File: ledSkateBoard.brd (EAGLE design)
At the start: 24.9 x 43.3 mm, 14 parts, among them J1 JST, U2 USD-SOCKETNEW, U4 MIC2505 3.3

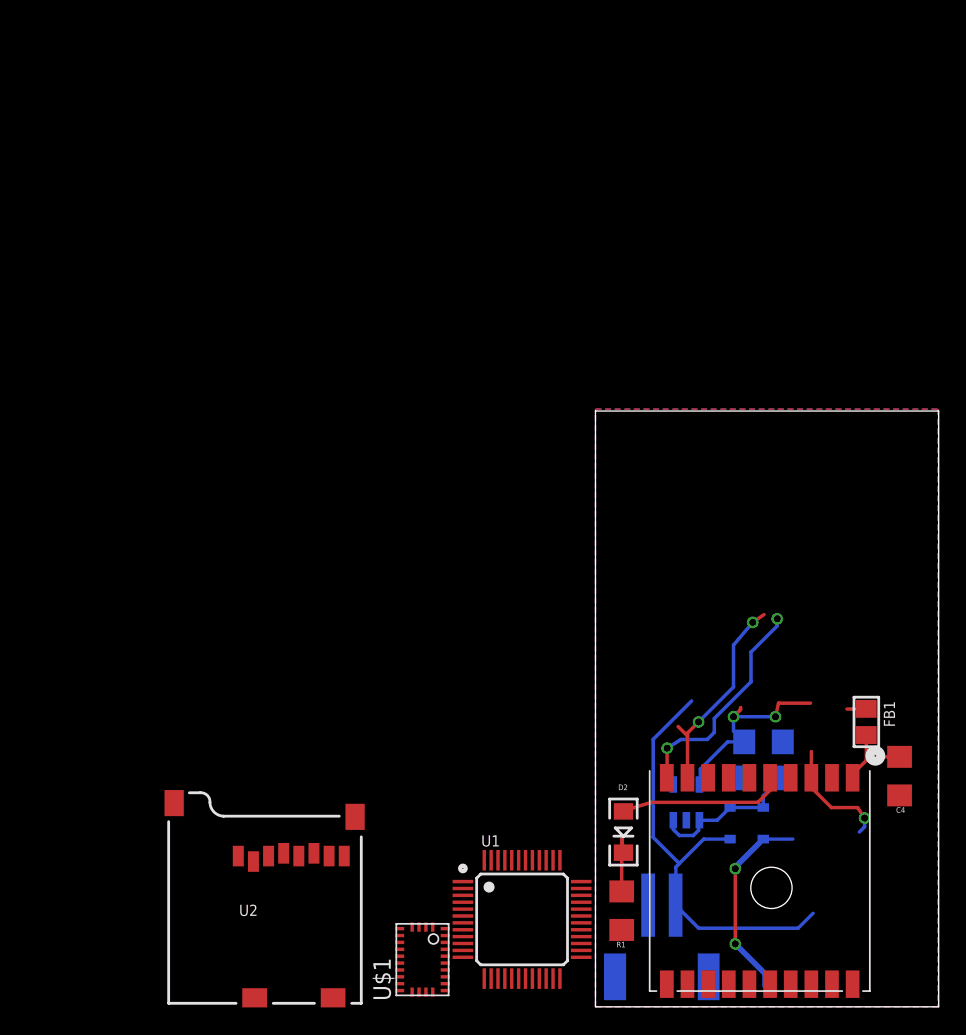
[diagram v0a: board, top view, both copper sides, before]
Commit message: faileld attempt
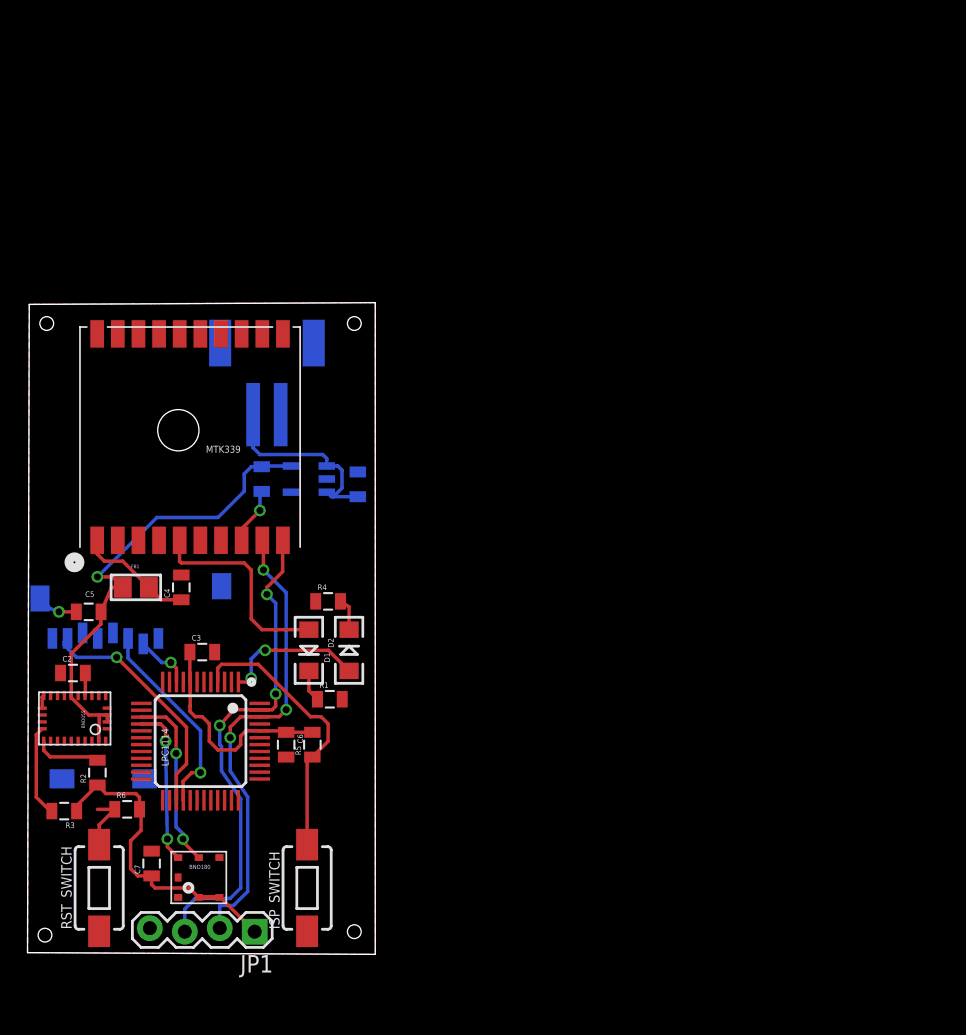
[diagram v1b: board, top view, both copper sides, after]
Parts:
- removed D3, D4: PMEG4005EJ, SparkFun-DiscreteSemi:SOD-323
- removed U1: (no value), microbuilder:LQFP48
- removed U2: USD-SOCKETNEW, SparkFun-Connectors:MICRO-SD-SOCKET-PP
- removed U3: (no value), adafruit:FGPMMOPA6H
- added BNO055: BNO055A, BNO055:BNO055
- added BNO180: BMP180, SparkFun-Sensors:BMP180
- added C2, C3, C6, C7: 10uF, SparkFun-Passives:0805
- added C5: .1uF, SparkFun-Passives:0805
- added D1: PURPLE, SparkFun-LED:LED-1206
- added ISP_SWITCH, RST_SWITCH: (no value), SparkFun-Electromechanical:TACTILE-SWITCH-1101NE
- added JP1: (no value), SparkFun-Connectors:1X04_LOCK
- added LPC1114: (no value), microbuilder:LQFP48
- added MTK339: (no value), adafruit:FGPMMOPA6H
- added R2, R3, R5, R6: 10K, SparkFun-Passives:0805
- added R4: 330, SparkFun-Passives:0805
- C14, C15, C4: device SparkFun-Capacitors:1206 -> SparkFun-Passives:0805
- R1: device SparkFun-Passives:1206 -> SparkFun-Passives:0805
- U$1: value BNO055A -> MICROSD; device BNO055:BNO055 -> adafruit:MICROSD
- moved FB1 54.0 mm to (10.4, 30.0), turned to 180 degrees
- moved C4 54.0 mm to (13.7, 30.0), turned to 90 degrees
- moved J1 51.7 mm to (19.9, 46.2), turned to 0 degrees
- moved C15 41.2 mm to (19.6, 37.8), turned to 90 degrees
- moved C14 36.3 mm to (26.5, 37.5), turned to 270 degrees
- moved U4 36.1 mm to (23.0, 37.8), turned to 270 degrees
- moved U$1 30.9 mm to (3.05, 15.6), flipped to the bottom, turned to 180 degrees
- moved D2 26.4 mm to (23.0, 25.4)
- moved R1 26.2 mm to (24.5, 21.8), turned to 0 degrees
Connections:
- removed net 5V: D3.A
- removed net GPS_RX: U1.47, U3.P$10
- removed net GPS_TX: U1.46, U3.P$9
- removed net N$10: C14.2, D3.C, D4.C, U4.1, U4.3
- removed net VDD(3.3V): U1.44
- removed net VDD(IO): U1.8
- removed net VSS(IO): U1.5
- new net BNO_INT: BNO055.14, LPC1114.14
- new net ISP: ISP_SWITCH.2, LPC1114.4, R5.1
- new net LPC_RX: JP1.2, LPC1114.46, MTK339.P$9
- new net LPC_TX: JP1.3, LPC1114.47, MTK339.P$10
- new net N$1: D1.A, LPC1114.1
- new net N$2: BNO055.9, C2.2
- new net N$3: D1.C, R4.2
- new net RESET: LPC1114.3, R6.1, RST_SWITCH.2
- new net SCL: BNO055.19, BNO180.5, LPC1114.15, R3.2
- new net SDA: BNO055.20, BNO180.6, LPC1114.16, R2.2
- new net SD_CS: LPC1114.10, U$1.2
- new net SD_DETECT: U$1.CD1
- new net SD_DI: LPC1114.28, U$1.3
- new net SD_DO: LPC1114.27, U$1.7
- new net SD_SCK: LPC1114.22, U$1.5
- new net VDD: U$1.4
- net GND: now also BNO055.10, BNO055.15, BNO055.16, BNO055.17, BNO055.18, BNO055.2, BNO055.25, BNO055.5, BNO055.6, BNO180.7, C2.1, C3.2, C5.1, C6.2, C7.2, ISP_SWITCH.1, J1.1, JP1.4, LPC1114.41, LPC1114.5, MTK339.P$12, MTK339.P$19, MTK339.P$3, MTK339.P$8, R4.1, RST_SWITCH.1, U$1.MT1, U$1.MT2; no longer U3.P$19, U3.P$3, U3.P$8
- net N$4: now also MTK339.P$1; no longer U3.P$1
- net N$6: now also MTK339.P$5; no longer U3.P$5
- net VCC: now also BNO055.11, BNO055.28, BNO055.3, BNO055.4, BNO180.2, BNO180.3, C3.1, C5.2, C6.1, C7.1, JP1.1, LPC1114.44, LPC1114.8, R2.1, R3.1, R5.2, R6.2
- net VSS: now also U$1.6; no longer U1.41
- net V_BATT: now also C14.2, J1.2, U4.1, U4.3; no longer D4.A
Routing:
- net VCC: track 16.0 -> 74.8 mm, vias 2 -> 1
- net LPC_TX: track 0.00 -> 36.2 mm, vias 0 -> 3
- net LPC_RX: track 0.00 -> 34.1 mm, vias 0 -> 3
- net ISP: track 0.00 -> 20.4 mm
- net SCL: track 0.00 -> 19.7 mm, vias 0 -> 2
- net V_BATT: track 32.4 -> 14.5 mm
- net SD_DO: track 0.00 -> 17.6 mm, vias 0 -> 1
- net GPS_RX: track 16.8 -> 0.00 mm, vias 2 -> 0
- net SDA: track 0.00 -> 16.5 mm, vias 0 -> 2
- net GPS_TX: track 15.2 -> 0.00 mm, vias 2 -> 0
- net SD_DI: track 0.00 -> 14.9 mm, vias 0 -> 1
- net 5V: track 14.5 -> 0.00 mm, vias 2 -> 0
- net N$10: track 11.3 -> 0.00 mm
- net N$1: track 0.00 -> 10.4 mm, vias 0 -> 2
- net RESET: track 0.00 -> 4.29 mm
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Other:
- board size 24.9 x 43.3 mm -> 25.3 x 47.4 mm

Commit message: semi final version pending review
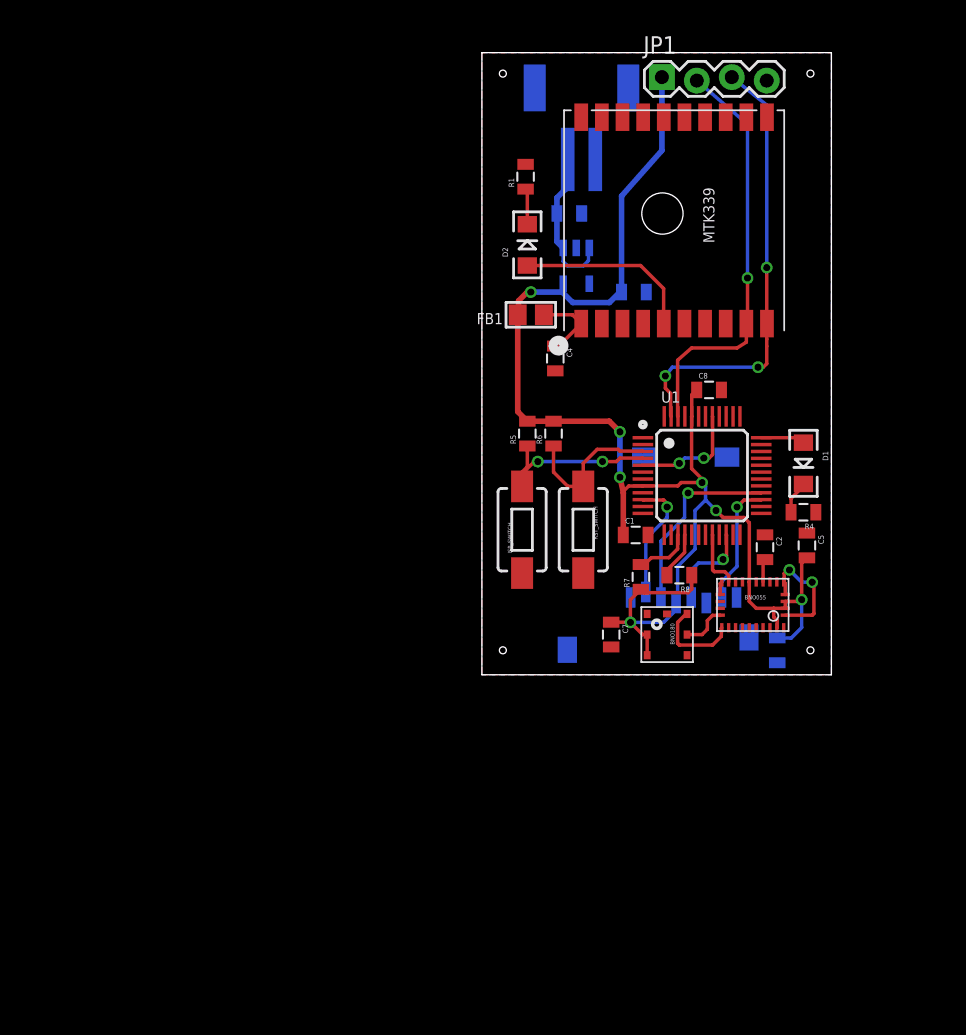
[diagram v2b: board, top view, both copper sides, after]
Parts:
- removed C6: 10uF, SparkFun-Passives:0805
- removed LPC1114: (no value), microbuilder:LQFP48
- removed R2, R3: 10K, SparkFun-Passives:0805
- removed U$1: MICROSD, adafruit:MICROSD
- added C1, C8: 10uF, SparkFun-Passives:0805
- added R7, R8: 10K, SparkFun-Passives:0805
- added SDCARD: MICROSD, adafruit:MICROSD
- added U1: (no value), microbuilder:LQFP48
- moved JP1 68.6 mm to (48.6, 66.9), turned to 0 degrees
- moved C5 52.4 mm to (59.2, 33.0), turned to 270 degrees
- moved C2 51.1 mm to (56.1, 32.9), turned to 270 degrees
- moved BNO055 50.0 mm to (55.2, 28.7)
- moved RST_SWITCH 43.8 mm to (42.9, 34.2)
- moved C3 41.8 mm to (57.0, 25.4), flipped to the bottom, turned to 90 degrees
- moved R6 41.3 mm to (40.8, 41.1), turned to 90 degrees
- moved R1 40.5 mm to (38.7, 59.8), turned to 90 degrees
- moved MTK339 38.5 mm to (49.5, 56.6)
- moved BNO180 38.3 mm to (49.0, 26.5), turned to 90 degrees
- moved C7 37.3 mm to (45.0, 26.5), turned to 270 degrees
- moved D1 35.7 mm to (58.9, 39.0), turned to 270 degrees
- moved R4 35.1 mm to (58.9, 35.4), turned to 180 degrees
- moved FB1 34.9 mm to (39.1, 49.8)
- moved D2 33.5 mm to (38.9, 54.9), turned to 90 degrees
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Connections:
- removed net VDD: U$1.4
- removed net VSS: U$1.6
- new net N$5: R8.2, U1.16
- new net N$7: R4.1
- new net N$8: R7.2, U1.15
- net BNO_INT: now also U1.20; no longer LPC1114.14
- net GND: now also C1.2, C3.1, C8.2, SDCARD.6, SDCARD.MT1, SDCARD.MT2, U1.41, U1.5; no longer C3.2, C6.2, LPC1114.41, LPC1114.5, R4.1, U$1.MT1, U$1.MT2
- net ISP: now also U1.4; no longer LPC1114.4
- net LPC_RX: now also U1.46; no longer LPC1114.46
- net LPC_TX: now also U1.47; no longer LPC1114.47
- net N$1: now also U1.36; no longer LPC1114.1
- net RESET: now also U1.3; no longer LPC1114.3
- net SCL: no longer LPC1114.15, R3.2
- net SDA: no longer LPC1114.16, R2.2
- net SD_CS: now also SDCARD.2, U1.10; no longer LPC1114.10, U$1.2
- net SD_DETECT: now also SDCARD.CD1; no longer U$1.CD1
- net SD_DI: now also SDCARD.3, U1.28; no longer LPC1114.28, U$1.3
- net SD_DO: now also SDCARD.7, U1.27; no longer LPC1114.27, U$1.7
- net SD_SCK: now also SDCARD.5, U1.22; no longer LPC1114.22, U$1.5
- net VCC: now also C1.1, C3.2, C8.1, R7.1, R8.1, SDCARD.4, U1.44, U1.8; no longer C3.1, C6.1, LPC1114.44, LPC1114.8, R2.1, R3.1
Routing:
- net VCC: track 74.8 -> 112.0 mm, vias 1 -> 7
- net SCL: track 19.7 -> 3.37 mm, vias 2 -> 0
- net SDA: track 16.5 -> 6.59 mm, vias 2 -> 0
- net GND: track 8.10 -> 17.7 mm, vias 2 -> 4
- net SD_DO: track 17.6 -> 9.03 mm
- net ISP: track 20.4 -> 12.7 mm, vias 0 -> 2
- net N$1: track 10.4 -> 3.22 mm, vias 2 -> 0
- net RESET: track 4.29 -> 11.0 mm
- net SD_SCK: track 0.00 -> 6.53 mm, vias 0 -> 1
- net SD_CS: track 4.15 -> 8.95 mm
- net BNO_INT: track 0.00 -> 4.37 mm
- net N$8: track 0.00 -> 4.18 mm
- net LPC_RX: track 34.1 -> 30.3 mm, vias 3 -> 1
- net N$5: track 0.00 -> 3.48 mm
- net V_BATT: track 14.5 -> 11.1 mm
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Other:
- board size 25.3 x 47.4 mm -> 25.4 x 45.2 mm
